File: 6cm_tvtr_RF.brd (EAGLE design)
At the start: 147 x 53 mm, 26 parts

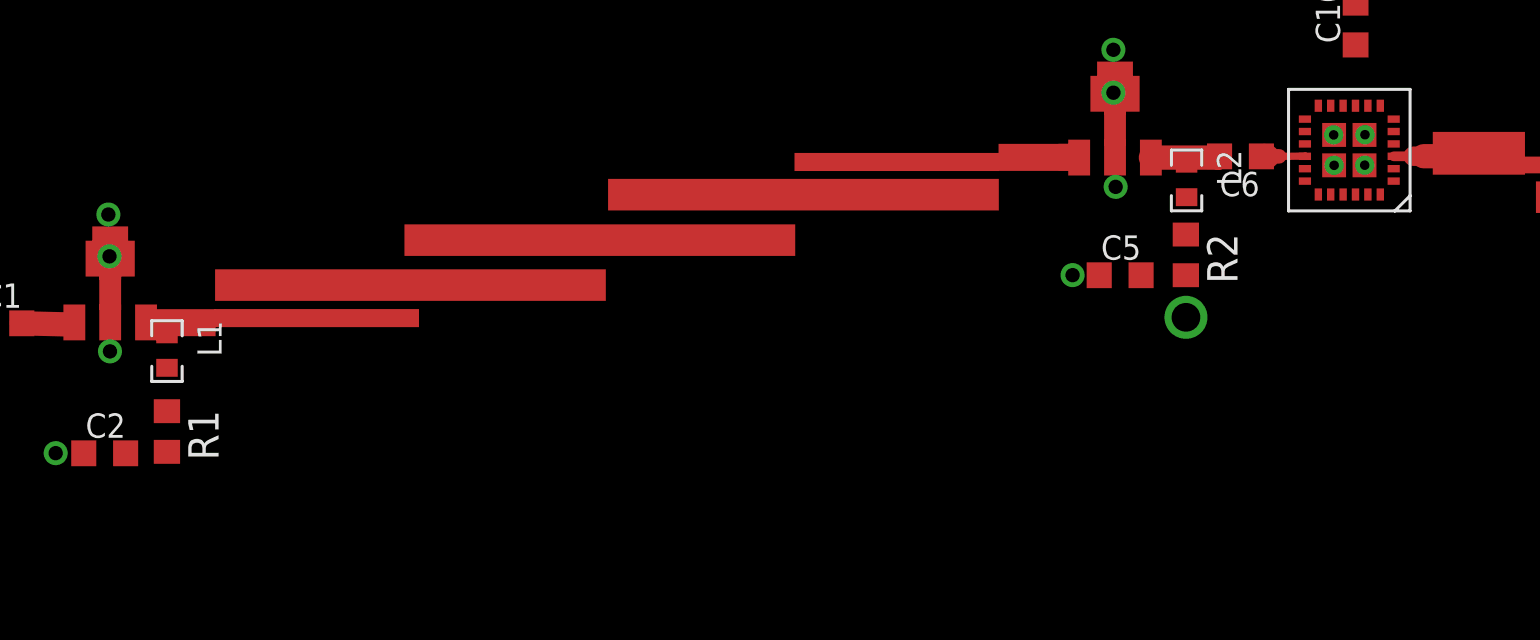
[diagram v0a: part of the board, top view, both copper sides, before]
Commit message: misc
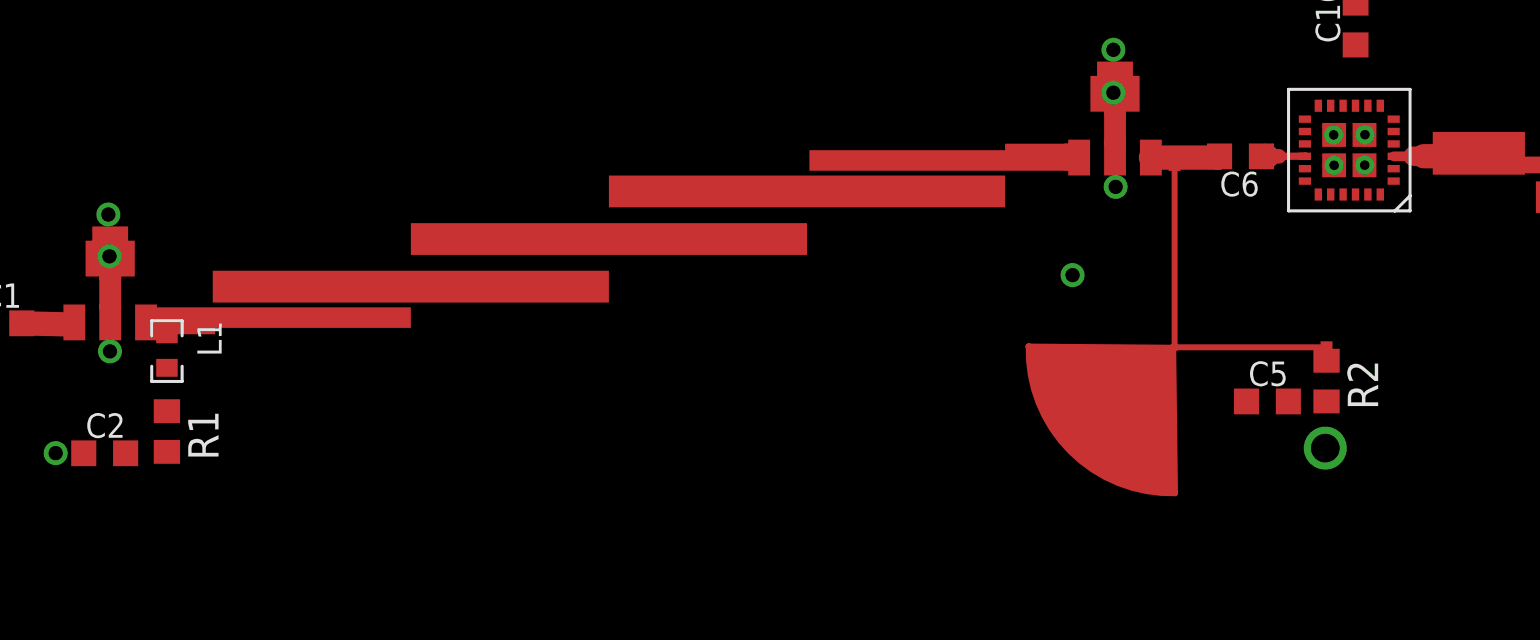
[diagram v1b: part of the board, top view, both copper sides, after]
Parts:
- removed L2: 0603, inductors:0603
- added U$9: STUB, microstrip:5.3_R4350B_508_STUB_90
- U$5: value 5_32_BP_ISOL -> 5_32_BP_ISOL532_R4350B_508_3EC; device microstrip:532_R4003C_508_3EC -> microstrip:532_R4350B_508_3EC
- moved C5 8.11 mm to (57.1, 24.7)
- moved R2 7.90 mm to (59.6, 25.6)
- moved U$5 1.23 mm to (46.2, 35.2)
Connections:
- net N$2: now also U$9.DC; no longer L2.P$2
- net N$3: now also U$9.RF; no longer L2.P$1
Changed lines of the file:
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@@
 <element name="C1" library="rcl" package="C0603K" value="" x="4.173984375" y="27.99445625"/>
 <element name="L1" library="inductors" package="0603" value="0603" x="11.11834375" y="26.83424375" rot="R270"/>
-<element name="R2" library="resistor" package="R0603" value="" x="53.70956875" y="30.855678125" rot="R270"/>
-<element name="C5" library="rcl" package="C0603K" value="" x="50.963084375" y="30.004790625"/>
+<element name="R2" library="resistor" package="R0603" value="" x="59.589678125" y="25.57913125" rot="R270"/>
+<element name="C5" library="rcl" package="C0603K" value="" x="57.1196" y="24.72824375"/>
 <element name="C6" library="rcl" package="C0603K" value="" x="55.993453125" y="34.97316875" rot="R180"/>
-<element name="U$5" library="microstrip" package="532_R4003C_508_3EC" value="5_32_BP_ISOL" x="45.892409375" y="34.032375" rot="R180"/>
+<element name="U$5" library="microstrip" package="532_R4350B_508_3EC" value="5_32_BP_ISOL532_R4350B_508_3EC" x="46.152590625" y="35.23255625" rot="R180"/>
 <element name="U$6" library="microstrip" package="576_R403C_508_5TH" value="5_7_GHZ_BP_ISOL" x="68.343315625" y="32.60776875"/>
 <element name="U$8" library="microstrip" package="DG1847" value="MDB-73H+" x="60.54223125" y="35.2346375" rot="R180"/>
 <element name="R1" library="resistor" package="R0603" value="" x="11.11649375" y="23.4717625" rot="R270"/>
-<element name="L2" library="inductors" package="0603" value="0603" x="53.740178125" y="33.96745625" rot="R270"/>
 <element name="C2" library="rcl" package="C0603K" value="" x="8.51499375" y="22.561515625"/>
 <element name="U$1" library="RF" package="DF782" value="GALI39+" x="8.7443375" y="28.032375"/>
@@
 <element name="L4" library="inductors" package="0603" value="0603" x="141.036853125" y="28.5884" rot="R90"/>
 <element name="C10" library="rcl" package="C0603K" value="" x="60.8061875" y="40.50694375" rot="R90"/>
+<element name="U$9" library="microstrip" package="5.3_R4350B_508_STUB_90" value="STUB" x="53.239759375" y="26.9927125" rot="R180"/>
 </elements>
 <signals>
@@
 <wire x1="50.748609375" y1="34.92323125" x2="50.748609375" y2="36.19323125" width="0" layer="19" extent="1-1"/>
 <wire x1="50.7756" y1="33.699334375" x2="50.748609375" y2="34.92323125" width="0" layer="19" extent="1-1"/>
-<wire x1="50.088084375" y1="30.004790625" x2="50.7756" y2="33.699334375" width="0" layer="19" extent="1-1"/>
-<wire x1="48.97415625" y1="30.009290625" x2="50.088084375" y2="30.004790625" width="0" layer="19" extent="1-1"/>
+<wire x1="56.2446" y1="24.72824375" x2="50.7756" y2="33.699334375" width="0" layer="19" extent="1-1"/>
+<wire x1="48.97415625" y1="30.009290625" x2="56.2446" y2="24.72824375" width="0" layer="19" extent="1-1"/>
 <wire x1="9.3158375" y1="30.699375" x2="48.97415625" y2="30.009290625" width="0" layer="19" extent="1-1"/>
 <wire x1="8.7443375" y1="30.572375" x2="9.3158375" y2="30.699375" width="0" layer="19" extent="1-1"/>
@@
 <contactref element="R2" pad="2"/>
 <contactref element="C5" pad="2"/>
-<via x="53.714375" y="28.245409375" extent="1-16" drill="1.2"/>
+<via x="59.539203125" y="22.778021875" extent="1-16" drill="1.2"/>
 <contactref element="R3" pad="2"/>
 <contactref element="C8" pad="2"/>
@@
 <wire x1="130.043640625" y1="35.05416875" x2="141.04091875" y2="35.176540625" width="0" layer="19" extent="1-1"/>
 <wire x1="130.031778125" y1="32.560471875" x2="130.043640625" y2="35.05416875" width="0" layer="19" extent="1-1"/>
-<wire x1="53.70956875" y1="30.005678125" x2="130.031778125" y2="32.560471875" width="0" layer="19" extent="1-1"/>
-<wire x1="51.838084375" y1="30.004790625" x2="53.70956875" y2="30.005678125" width="0" layer="19" extent="1-1"/>
-<wire x1="53.714375" y1="28.245409375" x2="53.70956875" y2="30.005678125" width="0" layer="19" extent="1-1"/>
+<wire x1="59.589678125" y1="24.72913125" x2="130.031778125" y2="32.560471875" width="0" layer="19" extent="1-1"/>
+<wire x1="57.9946" y1="24.72824375" x2="59.589678125" y2="24.72913125" width="0" layer="19" extent="1-1"/>
+<wire x1="59.539203125" y1="22.778021875" x2="59.589678125" y2="24.72913125" width="0" layer="19" extent="1-1"/>
 </signal>
 <signal name="N$5">
@@
 <contactref element="U$1" pad="P$3"/>
 <contactref element="L1" pad="P$1"/>
-<wire x1="10.2429375" y1="28.032375" x2="10.402115625" y2="28.0195125" width="0" layer="19" extent="1-1"/>
-<wire x1="11.11834375" y1="27.53424375" x2="10.402115625" y2="28.0195125" width="0" layer="19" extent="1-1"/>
+<wire x1="10.2429375" y1="28.032375" x2="10.407315625" y2="28.090225" width="0" layer="19" extent="1-1"/>
+<wire x1="11.11834375" y1="27.53424375" x2="10.407315625" y2="28.090225" width="0" layer="19" extent="1-1"/>
 </signal>
 <signal name="N$6">
 <contactref element="U$5" pad="P$2"/>
 <contactref element="U$2" pad="P$1"/>
-<wire x1="49.250009375" y1="34.92323125" x2="48.62738125" y2="34.933003125" width="0" layer="19" extent="1-1"/>
+<wire x1="49.250009375" y1="34.92323125" x2="48.867640625" y2="34.945046875" width="0" layer="19" extent="1-1"/>
 </signal>
 <signal name="N$9">
@@
 <signal name="N$2">
 <contactref element="R2" pad="1"/>
-<contactref element="L2" pad="P$2"/>
-<wire x1="53.70956875" y1="31.705678125" x2="53.740178125" y2="33.26745625" width="0" layer="19" extent="1-1"/>
+<contactref element="U$9" pad="DC"/>
+<wire x1="59.589759375" y1="26.9927125" x2="59.589678125" y2="26.42913125" width="0" layer="19" extent="1-1"/>
 </signal>
 <signal name="VCC">
@@
 <signal name="N$3">
 <contactref element="U$2" pad="P$3"/>
-<contactref element="L2" pad="P$1"/>
 <contactref element="C6" pad="2"/>
 <wire x1="52.247209375" y1="34.92323125" x2="55.068515625" y2="34.92323125" width="1.016" layer="1"/>
 <wire x1="55.068515625" y1="34.92323125" x2="55.118453125" y2="34.97316875" width="1.016" layer="1"/>
-<wire x1="55.068515625" y1="34.92323125" x2="53.740178125" y2="34.66745625" width="0" layer="19" extent="1-1"/>
+<contactref element="U$9" pad="RF"/>
+<wire x1="53.239759375" y1="21.9127125" x2="52.247209375" y2="34.92323125" width="0" layer="19" extent="1-1"/>
 </signal>
 <signal name="N$7">
